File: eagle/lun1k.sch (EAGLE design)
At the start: 100 parts, among them IC1 LTC3558, IC3 STM32F405RGT, IC4 NRF24L01SMD, J2 XF2-3015-1LW, Q1 Q12M-SMD-S, Q2 3.2X2.5CRYSTAL, SW1 JS102011SAQN, SW2 SWITCH_MCTAEF, SW3 SWITCH_MCTAEF, SW4 SWITCH_MCTAEF, T5 SI2301DS, T6 SI2301DS, U1 N35P112, X1 MICROUSB, X1_ JST-PH3

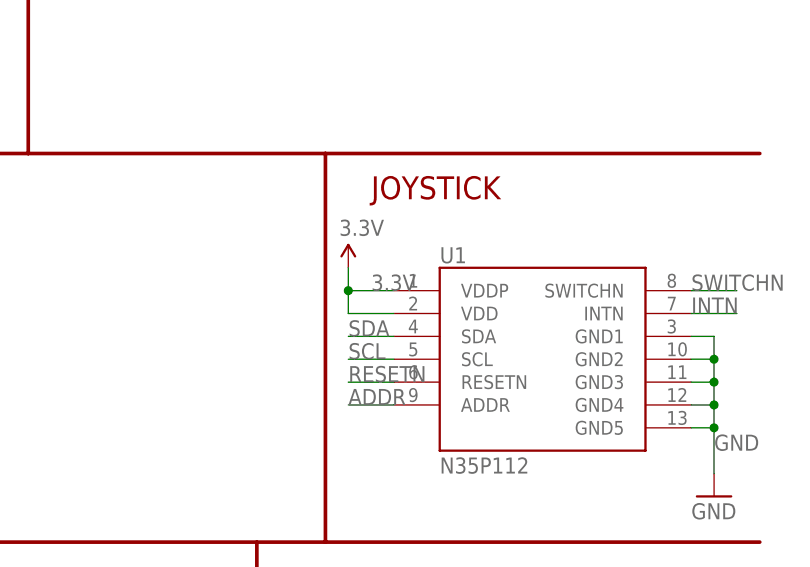
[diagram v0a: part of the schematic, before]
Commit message: routing
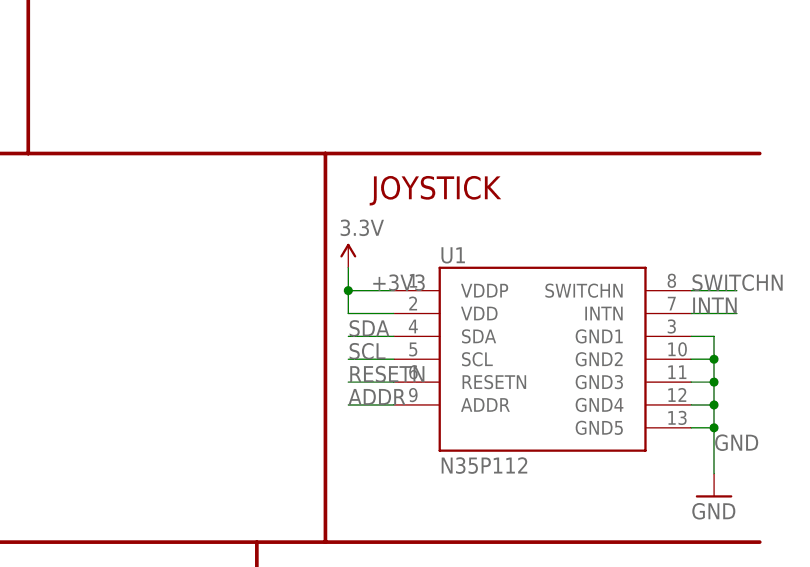
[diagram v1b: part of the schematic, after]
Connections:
- net +3V3: now also C11.2, C12.2, L5.2, R32.2, U1.VDD, U1.VDDP
- net 3.3V: no longer C11.2, C12.2, L5.2, R32.2, U1.VDD, U1.VDDP
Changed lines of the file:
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@@
 <pinref part="+3V10" gate="G$1" pin="+3V3"/>
+</segment>
+<segment>
+<wire x1="584.2" y1="71.12" x2="594.36" y2="71.12" width="0.1524" layer="91"/>
+<wire x1="594.36" y1="71.12" x2="604.52" y2="71.12" width="0.1524" layer="91"/>
+<wire x1="604.52" y1="71.12" x2="604.52" y2="76.2" width="0.1524" layer="91"/>
+<wire x1="574.04" y1="71.12" x2="584.2" y2="71.12" width="0.1524" layer="91"/>
+<junction x="584.2" y="71.12"/>
+<junction x="594.36" y="71.12"/>
+<junction x="604.52" y="71.12"/>
+<pinref part="R32" gate="G$1" pin="2"/>
+<pinref part="C11" gate="G$1" pin="2"/>
+<pinref part="C12" gate="G$1" pin="2"/>
+<pinref part="L5" gate="G$1" pin="2"/>
+<pinref part="P+4" gate="G$1" pin="3.3V"/>
+</segment>
+<segment>
+<wire x1="342.9" y1="149.86" x2="342.9" y2="147.32" width="0.1524" layer="91"/>
+<wire x1="342.9" y1="147.32" x2="347.98" y2="147.32" width="0.1524" layer="91"/>
+<wire x1="347.98" y1="144.78" x2="342.9" y2="144.78" width="0.1524" layer="91"/>
+<wire x1="342.9" y1="144.78" x2="342.9" y2="147.32" width="0.1524" layer="91"/>
+<junction x="342.9" y="147.32"/>
+<label x="345.44" y="147.32" size="1.778" layer="95"/>
+<pinref part="P+8" gate="G$1" pin="3.3V"/>
+<pinref part="U1" gate="G$1" pin="VDDP"/>
+<pinref part="U1" gate="G$1" pin="VDD"/>
 </segment>
 </net>
@@
 <net name="3.3V" class="0">
 <segment>
-<wire x1="342.9" y1="149.86" x2="342.9" y2="147.32" width="0.1524" layer="91"/>
-<wire x1="342.9" y1="147.32" x2="347.98" y2="147.32" width="0.1524" layer="91"/>
-<wire x1="347.98" y1="144.78" x2="342.9" y2="144.78" width="0.1524" layer="91"/>
-<wire x1="342.9" y1="144.78" x2="342.9" y2="147.32" width="0.1524" layer="91"/>
-<junction x="342.9" y="147.32"/>
-<label x="345.44" y="147.32" size="1.778" layer="95"/>
-<pinref part="P+8" gate="G$1" pin="3.3V"/>
-<pinref part="U1" gate="G$1" pin="VDDP"/>
-<pinref part="U1" gate="G$1" pin="VDD"/>
-</segment>
-<segment>
 <wire x1="444.5" y1="177.8" x2="444.5" y2="175.26" width="0.1524" layer="91"/>
 <wire x1="444.5" y1="175.26" x2="444.5" y2="172.72" width="0.1524" layer="91"/>
@@
 <label x="426.72" y="116.84" size="1.778" layer="95" font="vector"/>
 </segment>
-<segment>
-<wire x1="584.2" y1="71.12" x2="594.36" y2="71.12" width="0.1524" layer="91"/>
-<wire x1="594.36" y1="71.12" x2="604.52" y2="71.12" width="0.1524" layer="91"/>
-<wire x1="604.52" y1="71.12" x2="604.52" y2="76.2" width="0.1524" layer="91"/>
-<wire x1="574.04" y1="71.12" x2="584.2" y2="71.12" width="0.1524" layer="91"/>
-<junction x="584.2" y="71.12"/>
-<junction x="594.36" y="71.12"/>
-<junction x="604.52" y="71.12"/>
-<pinref part="R32" gate="G$1" pin="2"/>
-<pinref part="C11" gate="G$1" pin="2"/>
-<pinref part="C12" gate="G$1" pin="2"/>
-<pinref part="L5" gate="G$1" pin="2"/>
-<pinref part="P+4" gate="G$1" pin="3.3V"/>
-</segment>
-</net>
+</net>
